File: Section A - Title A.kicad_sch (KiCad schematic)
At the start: 35 parts, among them U1 AD7190WBRUZ, Y1 ABC2-4.9152MHZ-4-T

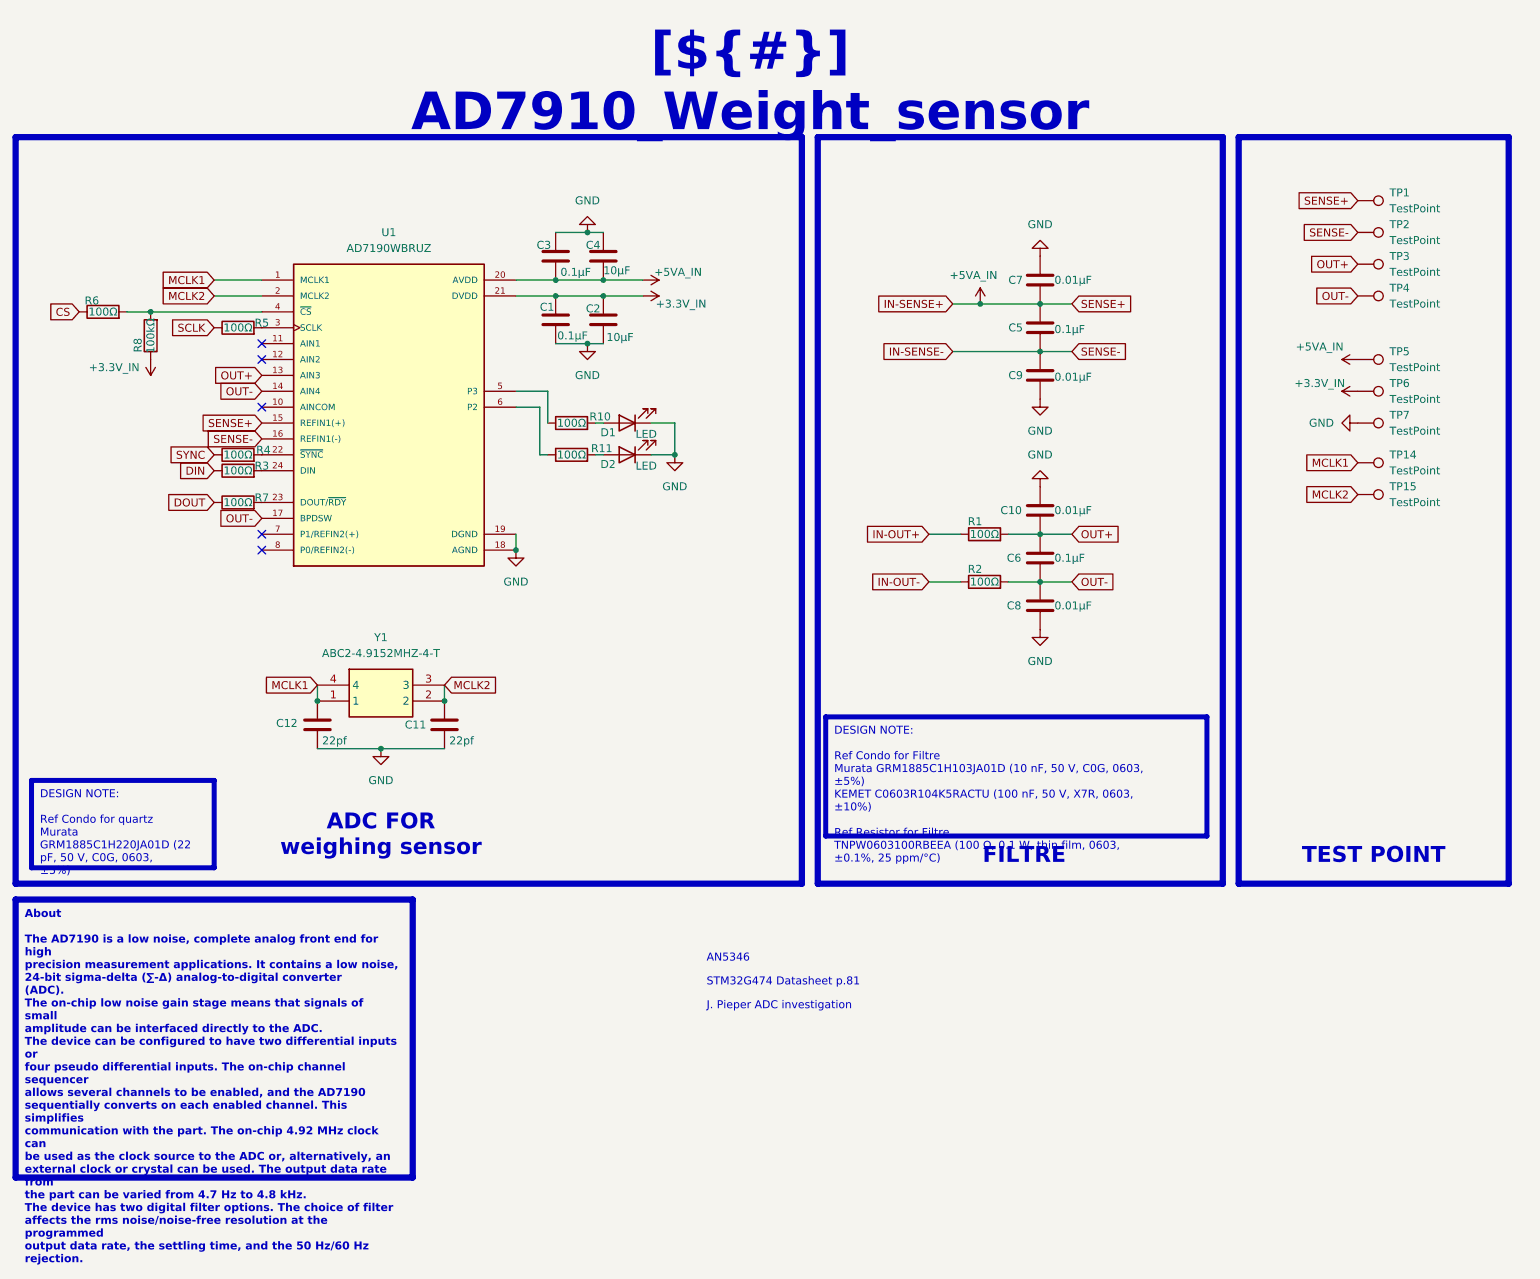
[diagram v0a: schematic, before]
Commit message: [PCB 4 layer]
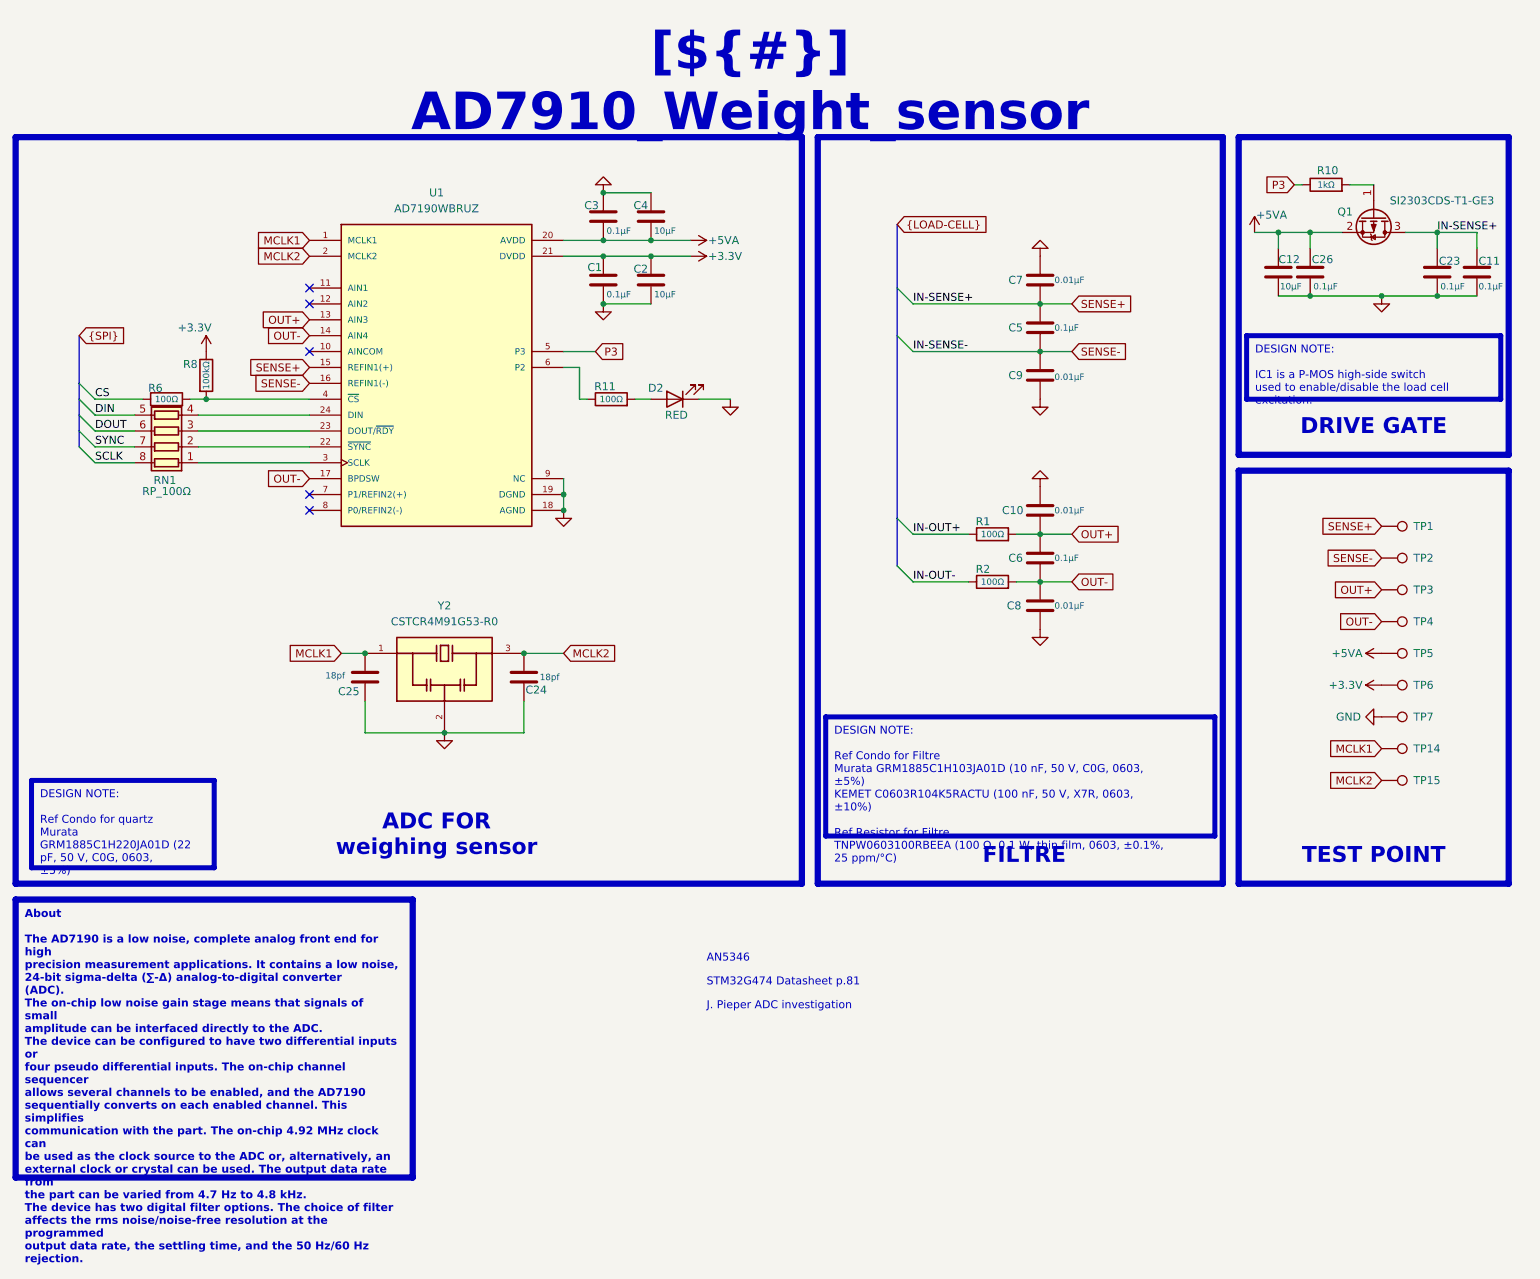
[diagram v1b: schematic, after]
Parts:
- removed D1: LED, LED_SMD:LED_0603_1608Metric, symbol Device:LED
- removed R3, R4, R5, R7: 100Ω, Resistor_SMD:R_0603_1608Metric, symbol Device:R
- removed Y1: ABC2-4.9152MHZ-4-T, ABC2-4.9152MHZ-4-T:ABC210000MHZ4, symbol ABC2-4_9152MHZ-4-T:ABC2-4.9152MHZ-4-T
- added C23, C26: 0.1µF, Capacitor_SMD:C_0603_1608Metric, symbol Device:C
- added C24, C25: 18pf, Capacitor_SMD:C_0603_1608Metric, symbol Device:C
- added Q1: SI2303CDS-T1-GE3, Package_TO_SOT_SMD:SOT-23-3, symbol Transistor_FET:CSD25480F3
- added RN1: RP_100Ω, Resistor_SMD:R_Array_Concave_4x0603, symbol Device:R_Pack04
- added Y2: CSTCR4M91G53-R0, CSTCR4M91G53-R0:OSC_CSTCR4M91G53-R0, symbol CSTCR4M91G53-R0:CSTCR4M91G53-R0
- C11: value 22pf -> 0.1µF
- C12: value 22pf -> 10µF
- D2: value LED -> RED
- R10: value 100Ω -> 1kΩ
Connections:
- net DIN: now also RN1.5 (R4.2)
- net DOUT: now also RN1.6 (R3.2)
- net GND: now also U1.9 (NC), C23.2, C24.2, C25.2, C26.2, Y2.2
- net MCLK1: now also C25.1, Y2.1; no longer C12.1
- net MCLK2: now also C24.1, Y2.3; no longer C11.1
- net SCLK: now also RN1.8 (R1.2)
- net SYNC: now also RN1.7 (R2.2)
- net at U1.3 (SCLK): now also RN1.1 (R1.1)
- net P3: now reaches R10.1, U1.5 (P3)
- net at R10.2: now also Q1.1 (G)
- net at U1.24 (DIN): now also RN1.4 (R4.1)
- net at U1.22 (~{SYNC}): now also RN1.2 (R2.1)
- net at U1.23 (DOUT/~{RDY}): now also RN1.3 (R3.1)
- net +3.3V_IN renamed +3.3V
- net +5VA_IN renamed +5VA
- net +5VA: now also C12.1, C26.1, Q1.2 (S); no longer C5.1, C7.2, TP1.1, U1.15 (REFIN1(+))
- net IN-SENSE- renamed SENSE-
- new net SENSE+: C11.1, C23.1, C5.1, C7.2, Q1.3 (D), TP1.1, U1.15 (REFIN1(+))
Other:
- moved on the sheet: C1, C2, C3, C4, D2, R1, R11, R2, R6, R8, TP1, TP14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
